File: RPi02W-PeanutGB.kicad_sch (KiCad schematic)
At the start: 58 parts, among them J1 Raspberry_Pi_2_3, J3 AudioJack3_SwitchTR, J4 Conn_01x50, J5 Conn_02x10_Odd_Even, J6 Conn_02x10_Odd_Even, J7 Conn_02x10_Odd_Even, J8 Conn_02x10_Odd_Even, J9 USB_C_Receptacle, SW1 SW_SPDT_MSM, SW10 SW_Push, SW11 SW_Push, SW12 SW_Push, SW13 SW_Push, SW14 SW_Push, SW2 SW_Push, SW3 SW_Push, SW4 SW_Push, SW5 SW_Push, SW6 SW_Push, SW7 SW_Push, SW8 SW_Push, SW9 SW_Push, U1 MCP73831-2-OT, U3 LM4861MX

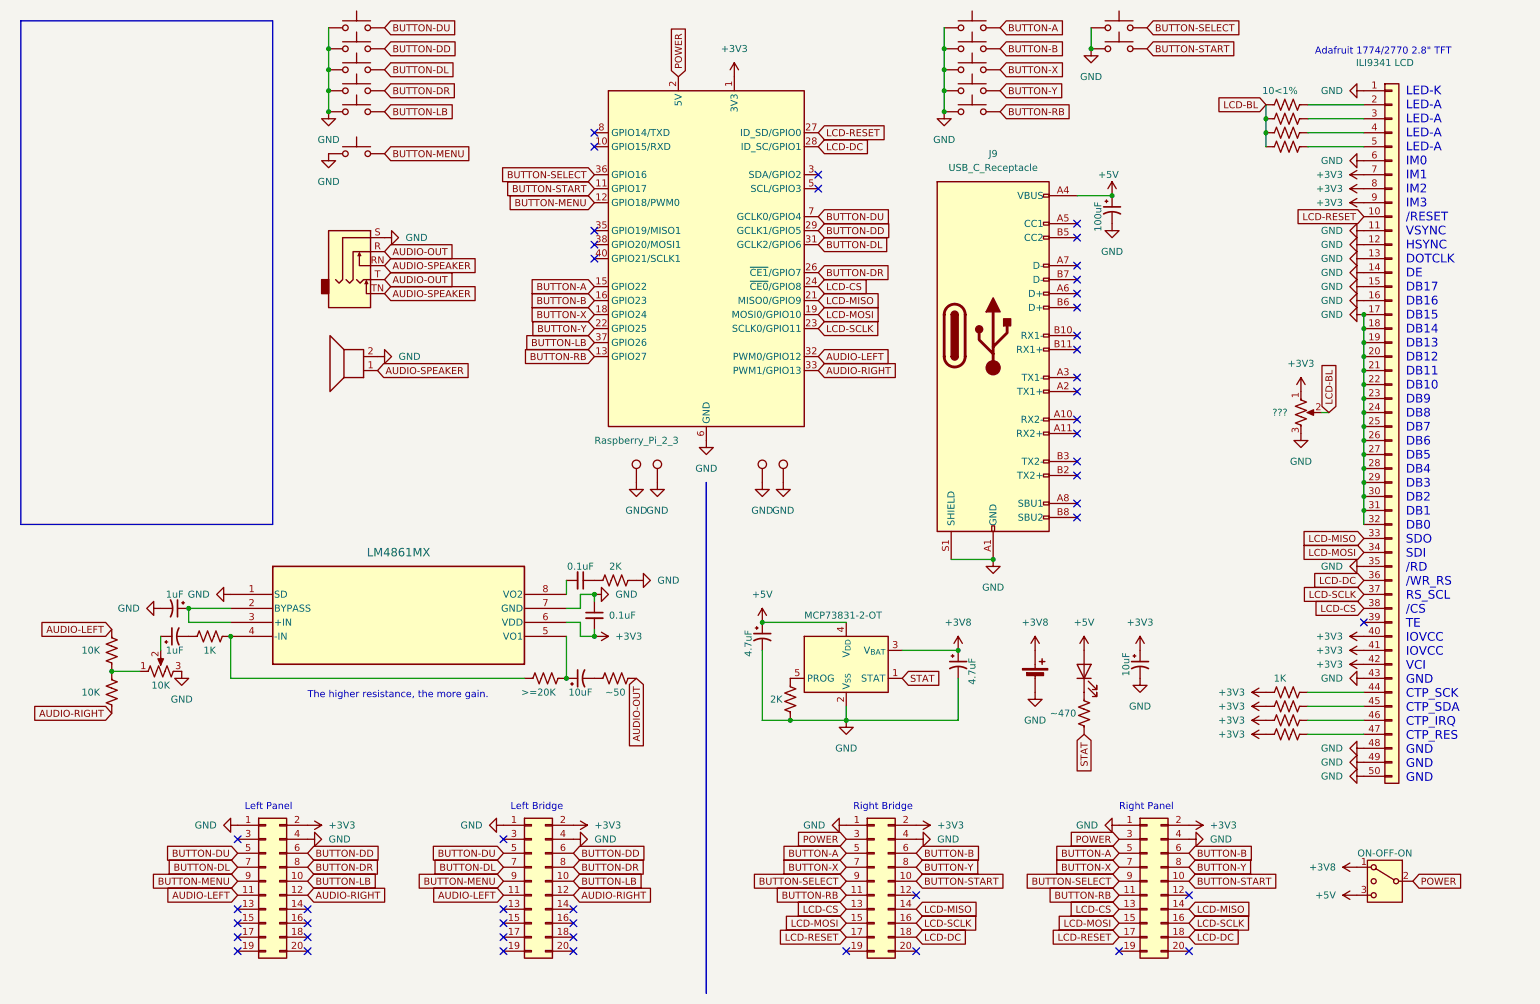
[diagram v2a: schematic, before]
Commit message: Add files via upload
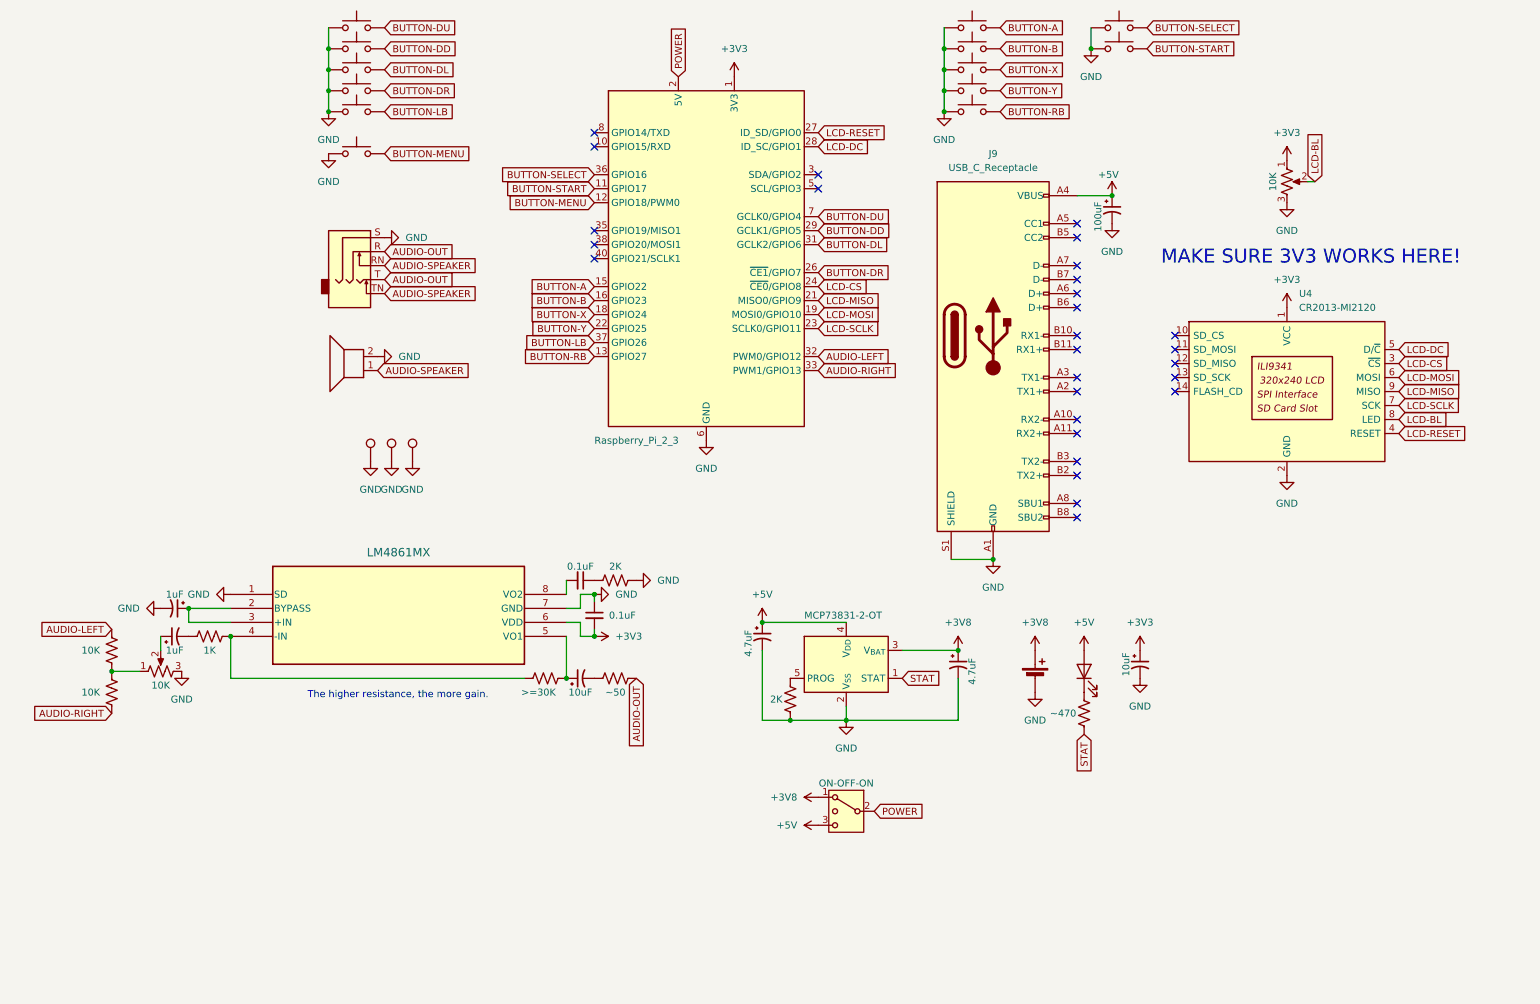
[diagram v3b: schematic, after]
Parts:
- removed J4: Conn_01x50, Connector_FFC-FPC:Hirose_FH12-50S-0.5SH_1x50-1MP_P0.50mm_Horizontal, symbol Connector_Generic:Conn_01x50
- removed J5, J6, J7, J8: Conn_02x10_Odd_Even, Connector_PinHeader_2.54mm:PinHeader_2x10_P2.54mm_Vertical, symbol Connector_Generic:Conn_02x10_Odd_Even
- removed R10, R11, R12, R13, R14, R15, R16, R9: R_US, Resistor_THT:R_Axial_DIN0207_L6.3mm_D2.5mm_P10.16mm_Horizontal, symbol Device:R_US
- removed RV1: R_Potentiometer_US, Potentiometer_THT:Potentiometer_Piher_PT-10-V10_Vertical_Hole, symbol Device:R_Potentiometer_US
- removed TP4: TestPoint, RPi02W-PeanutGB:ScrewHole-4-40, symbol Connector:TestPoint
- added RV3: R_Potentiometer_US, Potentiometer_THT:Potentiometer_Bourns_PTV09A-2_Single_Horizontal, symbol Device:R_Potentiometer_US
- added U4: CR2013-MI2120, Display:CR2013-MI2120, symbol Driver_Display:CR2013-MI2120
- C1, C2, C3, C4, C5, C9: footprint Capacitor_THT:CP_Radial_D6.3mm_P2.50mm -> Capacitor_SMD:CP_Elec_4x5.8
- C6, C7: footprint Capacitor_THT:C_Disc_D3.0mm_W1.6mm_P2.50mm -> Capacitor_SMD:C_1206_3216Metric_Pad1.33x1.80mm_HandSolder
- C8: footprint Capacitor_THT:CP_Radial_D6.3mm_P2.50mm -> Capacitor_THT:CP_Radial_D8.0mm_P2.50mm
- R1, R2, R3, R4, R5, R7, R8: footprint Resistor_THT:R_Axial_DIN0207_L6.3mm_D2.5mm_P10.16mm_Horizontal -> Resistor_SMD:R_1206_3216Metric_Pad1.30x1.75mm_HandSolder
- R6: footprint Resistor_THT:R_Axial_DIN0207_L6.3mm_D2.5mm_P10.16mm_Horizontal -> Resistor_SMD:R_1206_3216Metric_Pad1.30x1.75mm_HandSolder; Field4 >=20K -> >=30K
- RV2: footprint RPi02W-PeanutGB:RK10J1xE -> Potentiometer_THT:Potentiometer_Bourns_PTV09A-2_Single_Horizontal
- TP1, TP2, TP3: footprint RPi02W-PeanutGB:ScrewHole-4-40 -> RPi02W-PeanutGB:ScrewHole-RPiZero
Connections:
- net +3V3: now also RV3.1, U4.1 (VCC)
- net GND: now also RV3.3, U4.2 (GND)
- net LCD-BL: now also RV3.2, U4.8 (LED)
- net LCD-CS: now also U4.3 (~{CS})
- net LCD-DC: now also U4.5 (D/~{C})
- net LCD-MISO: now also U4.9 (MISO)
- net LCD-MOSI: now also U4.6 (MOSI)
- net LCD-RESET: now also U4.4 (RESET)
- net LCD-SCLK: now also U4.7 (SCK)
- no-connect marks 48 -> 28
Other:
- note added: "MAKE SURE 3V3 WORKS HERE!"
- note removed: "Adafruit 1774/2770 2.8" TFT"
- note removed: "LED-K LED-A LED-A LED-A LED-A IM0 IM1 IM2 IM3 /RESET VSYNC HSYNC DOTCLK DE DB17 DB16 DB15 DB14 DB13 DB12 DB11 DB10 DB9 DB8 DB7 DB6 DB5 DB4 DB3 DB2 DB1 DB0 SDO SDI /RD /WR_RS RS_SCL /CS TE IOVCC IOVCC VCI GND CTP_SCK CTP_SDA CTP_IRQ CTP_RES GND GND GND"
- note removed: "Left Bridge"
- note removed: "Left Panel"
- note removed: "Right Bridge"
- note removed: "Right Panel"
